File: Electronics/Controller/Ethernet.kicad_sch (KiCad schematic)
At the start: 33 parts, among them J301 08B1-1X1T-06-F, U203 ASDMB-25.000MHZ-LC-T, U301 W5500

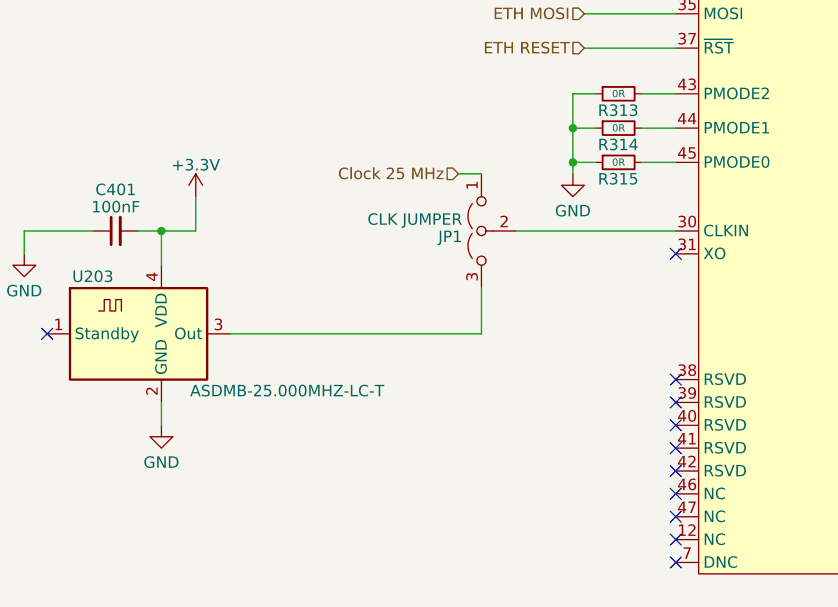
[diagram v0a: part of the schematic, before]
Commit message: Manufacturing Commit
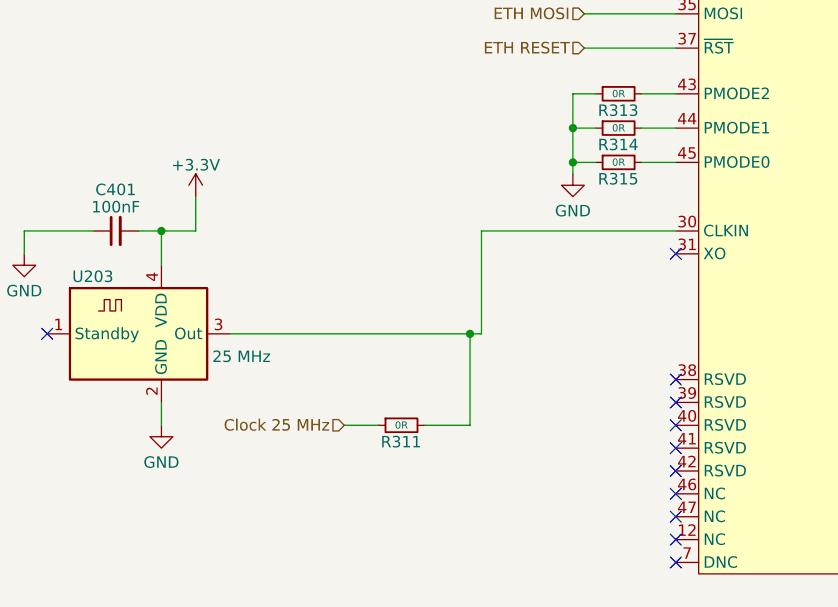
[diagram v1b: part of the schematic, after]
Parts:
- removed JP1: CLK JUMPER, Findersee_parts:0402_Jumper_3pin, symbol Jumper:Jumper_3_Open
- added R311: 0R, Resistor_SMD:R_0402_1005Metric, symbol Device:R_Small
- U203: value ASDMB-25.000MHZ-LC-T -> 25 MHz; footprint Oscillator:Oscillator_SMD_Abracon_ASDMB-4Pin_2.5x2.0mm -> Oscillator:Oscillator_SMD_SeikoEpson_SG8002CE-4Pin_3.2x2.5mm; Manufacturer Abracon -> (none)
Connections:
- net Clock 25 MHz: now also R311.1
- net at U301.30 (XI): now also U203.3 (Out), R311.2
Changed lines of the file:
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@@
   (junction (at 78.74 63.5) (diameter 0) (color 0 0 0 0)
+  )
+  (junction (at 77.47 127) (diameter 0) (color 0 0 0 0)
   )
   (junction (at 213.36 58.42) (diameter 0) (color 0 0 0 0)
@@
     (stroke (width 0) (type default))
   )
+  (wire (pts (xy 77.47 137.16) (xy 77.47 127))
+    (stroke (width 0) (type default))
+  )
   (wire (pts (xy 189.23 123.19) (xy 189.23 125.73))
     (stroke (width 0) (type default))
@@
     (stroke (width 0) (type default))
   )
+  (wire (pts (xy 72.39 137.16) (xy 77.47 137.16))
+    (stroke (width 0) (type default))
+  )
   (wire (pts (xy 224.79 58.42) (xy 256.54 58.42))
     (stroke (width 0) (type default))
@@
     (stroke (width 0) (type default))
   )
-  (wire (pts (xy 78.74 127) (xy 78.74 121.92))
+  (wire (pts (xy 78.74 115.57) (xy 78.74 127))
     (stroke (width 0) (type default))
   )
@@
     (stroke (width 0) (type default))
   )
+  (wire (pts (xy 77.47 127) (xy 78.74 127))
+    (stroke (width 0) (type default))
+  )
   (wire (pts (xy 171.45 71.12) (xy 172.72 71.12))
     (stroke (width 0) (type default))
@@
     (stroke (width 0) (type default))
   )
-  (wire (pts (xy 76.2 109.22) (xy 78.74 109.22))
+  (wire (pts (xy 63.5 137.16) (xy 67.31 137.16))
     (stroke (width 0) (type default))
   )
@@
     (stroke (width 0) (type default))
   )
-  (wire (pts (xy 50.8 127) (xy 78.74 127))
+  (wire (pts (xy 50.8 127) (xy 77.47 127))
     (stroke (width 0) (type default))
   )
@@
     (stroke (width 0) (type default))
   )
-  (wire (pts (xy 82.55 115.57) (xy 100.33 115.57))
-    (stroke (width 0) (type default))
-  )
   (wire (pts (xy 171.45 110.49) (xy 175.26 110.49))
     (stroke (width 0) (type default))
@@
   )
   (wire (pts (xy 213.36 34.29) (xy 229.87 34.29))
+    (stroke (width 0) (type default))
+  )
+  (wire (pts (xy 78.74 115.57) (xy 100.33 115.57))
     (stroke (width 0) (type default))
   )
@@
     (effects (font (size 1.27 1.27)) (justify right))
   )
-  (hierarchical_label "Clock 25 MHz" (shape input) (at 76.2 109.22 180) (fields_autoplaced)
+  (hierarchical_label "Clock 25 MHz" (shape input) (at 63.5 137.16 180) (fields_autoplaced)
     (effects (font (size 1.27 1.27)) (justify right))
   )
@@
     )
   )
+  (symbol (lib_id "Device:R_Small") (at 69.85 137.16 90) (mirror x) (unit 1)
+    (in_bom no) (on_board yes) (dnp no)
+    (property "Reference" "R311" (at 69.8041 139.0246 90)
+      (effects (font (size 1.27 1.27)))
+    )
+    (property "Value" "0R" (at 69.85 137.16 90)
+      (effects (font (size 0.8 0.8)))
+    )
+    (property "Footprint" "Resistor_SMD:R_0402_1005Metric" (at 69.85 137.16 0)
+      (effects (font (size 1.27 1.27)) hide)
+    )
+    (property "Datasheet" "~" (at 69.85 137.16 0)
+      (effects (font (size 1.27 1.27)) hide)
+    )
+    (pin "1")
+    (pin "2")
+    (instances
+      (project "Controller"
+        (path "/a2ea94cb-4178-4727-9ac9-0e597b4a505d/5e10769e-2c76-442d-969e-a77f15adcbc3"
+          (reference "R311") (unit 1)
+        )
+      )
+    )
+  )
   (symbol (lib_id "power:+3.3V") (at 46.99 111.76 0) (unit 1)
     (in_bom yes) (on_board yes) (dnp no) (fields_autoplaced)
@@
       (effects (font (size 1.27 1.27)))
     )
-    (property "Value" "ASDMB-25.000MHZ-LC-T" (at 57.15 133.35 0)
-      (effects (font (size 1.27 1.27)))
-    )
-    (property "Footprint" "Oscillator:Oscillator_SMD_Abracon_ASDMB-4Pin_2.5x2.0mm" (at 40.64 127 0)
-      (effects (font (size 1.27 1.27)) hide)
-    )
-    (property "Datasheet" "https://abracon.com/Oscillators/ASDMB.pdf" (at 48.26 115.57 0)
-      (effects (font (size 1.27 1.27)) hide)
-    )
-    (property "Manufacturer" "Abracon" (at 40.64 127 0)
+    (property "Value" "25 MHz" (at 52.07 129.54 0)
+      (effects (font (size 1.27 1.27)))
+    )
+    (property "Footprint" "Oscillator:Oscillator_SMD_SeikoEpson_SG8002CE-4Pin_3.2x2.5mm" (at 40.64 127 0)
+      (effects (font (size 1.27 1.27)) hide)
+    )
+    (property "Datasheet" "" (at 48.26 115.57 0)
+      (effects (font (size 1.27 1.27)) hide)
+    )
+    (property "Manufacturer" "" (at 40.64 127 0)
       (effects (font (size 1.27 1.27)) hide)
     )
@@
         )
       )
-    )
-  )
-  (symbol (lib_id "Jumper:Jumper_3_Open") (at 78.74 115.57 90) (mirror x) (unit 1)
-    (in_bom yes) (on_board yes) (dnp no)
-    (property "Reference" "JP1" (at 76.6058 116.2137 90)
-      (effects (font (size 1.27 1.27)) (justify left))
-    )
-    (property "Value" "CLK JUMPER" (at 76.6058 114.2927 90)
-      (effects (font (size 1.27 1.27)) (justify left))
-    )
-    (property "Footprint" "Findersee_parts:0402_Jumper_3pin" (at 78.74 115.57 0)
-      (effects (font (size 1.27 1.27)) hide)
-    )
-    (property "Datasheet" "~" (at 78.74 115.57 0)
-      (effects (font (size 1.27 1.27)) hide)
-    )
-    (pin "1")
-    (pin "2")
-    (pin "3")
-    (instances
-      (project "Controller"
-        (path "/a2ea94cb-4178-4727-9ac9-0e597b4a505d/5e10769e-2c76-442d-969e-a77f15adcbc3"
-          (reference "JP1") (unit 1)
-        )
-      )
